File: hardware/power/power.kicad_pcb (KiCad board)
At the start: 2 copper layers, 37 x 41 mm, 30 parts, among them J1 SF6, J2 SF6, J3 PinHeader2x4, J4 PinHeader2x4, J5 PinHeader2x4, J6 SF6, J7 SF6, J8 SF6, Q1 ISC022N10NM6, Q2 ISC022N10NM6, Q3 ISC022N10NM6, Q4 ISC022N10NM6, Q5 ISC022N10NM6, Q6 ISC022N10NM6

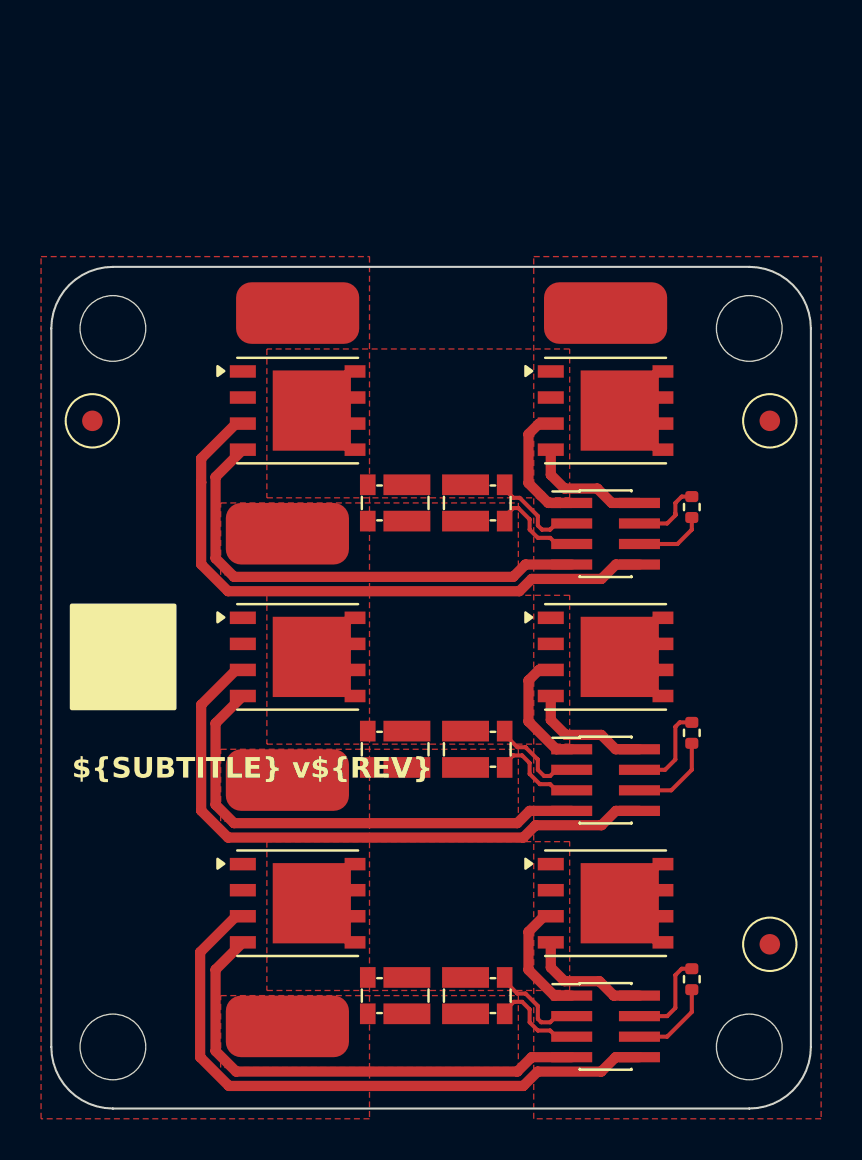
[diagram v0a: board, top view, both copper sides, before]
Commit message: intermediate commit, some changes needed before first purchase
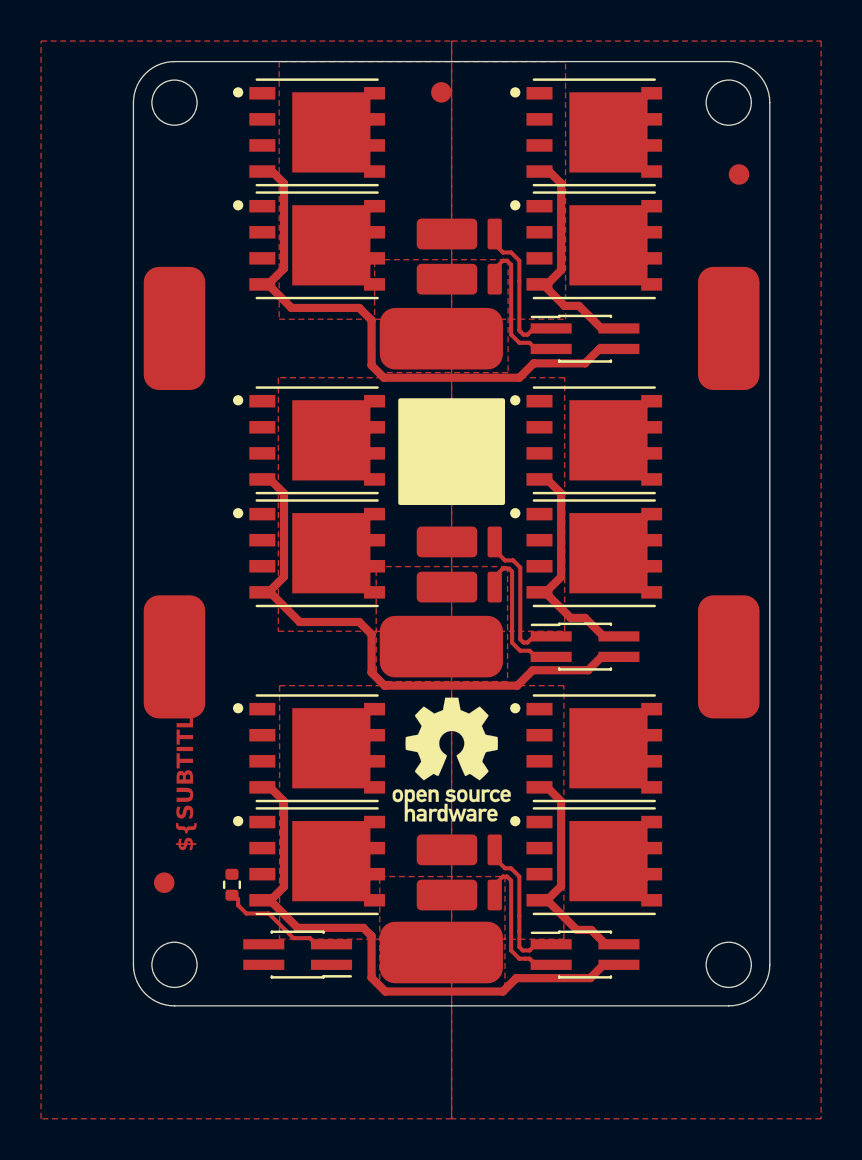
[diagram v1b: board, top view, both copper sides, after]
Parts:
- removed H1, H2, H3, H4: HoleM3_ISO14580, MountingHole:MountingHole_3.2mm_M3_ISO14580
- removed Q1, Q2, Q3, Q4, Q5, Q6: ISC022N10NM6, Package_SO:PowerPAK_SO-8_Single
- removed R2, R3, R4, R5, R6: 500u, Resistor_SMD:R_Shunt_Vishay_WSKW0612
- removed TH1, TH2, TH3: NTC 10k, Resistor_SMD:R_0402_1005Metric
- added H101: HoleM2_ISO14580, MountingHole:MountingHole_2.2mm_M2_ISO14580, F.Cu at (116.0, 42.0)
- added H102: HoleM2_ISO14580, MountingHole:MountingHole_2.2mm_M2_ISO14580, F.Cu at (89.0, 84.0)
- added H103: HoleM2_ISO14580, MountingHole:MountingHole_2.2mm_M2_ISO14580, F.Cu at (89.0, 42.0)
- added H104: HoleM2_ISO14580, MountingHole:MountingHole_2.2mm_M2_ISO14580, F.Cu at (116.0, 84.0)
- added J109: SF6, Connector_Wire:SolderWirePad_1x01_SMD_3x6mm, F.Cu at (116.0, 69.0)
- added J110: SF6, Connector_Wire:SolderWirePad_1x01_SMD_3x6mm, F.Cu at (89.0, 69.0)
- added J111: PinHeader2x2, Connector_PinHeader_1.00mm:PinHeader_2x02_P1.00mm_Vertical_SMD, F.Cu at (95.0, 83.5)
- added Q201: ISC022N10NM6, mcrmv:PowerPAK_SO-8_Single, F.Cu at (110.0, 43.5)
- added Q202: ISC022N10NM6, mcrmv:PowerPAK_SO-8_Single, F.Cu at (96.5, 43.5)
- added Q203: ISC022N10NM6, mcrmv:PowerPAK_SO-8_Single, F.Cu at (110.0, 58.5)
- added Q204: ISC022N10NM6, mcrmv:PowerPAK_SO-8_Single, F.Cu at (96.5, 58.5)
- added Q205: ISC022N10NM6, mcrmv:PowerPAK_SO-8_Single, F.Cu at (110.0, 73.5)
- added Q206: ISC022N10NM6, mcrmv:PowerPAK_SO-8_Single, F.Cu at (96.5, 73.5)
- added Q301: ISC022N10NM6, mcrmv:PowerPAK_SO-8_Single, F.Cu at (110.0, 49.0)
- added Q302: ISC022N10NM6, mcrmv:PowerPAK_SO-8_Single, F.Cu at (96.5, 49.0)
- added Q303: ISC022N10NM6, mcrmv:PowerPAK_SO-8_Single, F.Cu at (110.0, 64.0)
- added Q304: ISC022N10NM6, mcrmv:PowerPAK_SO-8_Single, F.Cu at (96.5, 64.0)
- added Q305: ISC022N10NM6, mcrmv:PowerPAK_SO-8_Single, F.Cu at (110.0, 79.0)
- added Q306: ISC022N10NM6, mcrmv:PowerPAK_SO-8_Single, F.Cu at (96.5, 79.0)
- added R102: 200u, mcrmv:WSK1216, F.Cu at (104.0, 64.5)
- added R103: 200u, mcrmv:WSK1216, F.Cu at (104.0, 79.5)
- added REF**: OSHW-Logo_5.7x6mm_SilkScreen, Symbol:OSHW-Logo_5.7x6mm_SilkScreen, F.Cu at (102.5, 74.0)
- added TH101: NTC 10k, Resistor_SMD:R_0402_1005Metric, F.Cu at (91.8, 80.1)
- J103: renamed from J3; value PinHeader2x4 -> PinHeader2x2; footprint Connector_PinHeader_1.00mm:PinHeader_2x04_P1.00mm_Vertical_SMD -> Connector_PinHeader_1.00mm:PinHeader_2x02_P1.00mm_Vertical_SMD
- J104: renamed from J4; value PinHeader2x4 -> PinHeader2x2; footprint Connector_PinHeader_1.00mm:PinHeader_2x04_P1.00mm_Vertical_SMD -> Connector_PinHeader_1.00mm:PinHeader_2x02_P1.00mm_Vertical_SMD
- J105: renamed from J5; value PinHeader2x4 -> PinHeader2x2; footprint Connector_PinHeader_1.00mm:PinHeader_2x04_P1.00mm_Vertical_SMD -> Connector_PinHeader_1.00mm:PinHeader_2x02_P1.00mm_Vertical_SMD
- R101: renamed from R1; value 500u -> 200u; footprint Resistor_SMD:R_Shunt_Vishay_WSKW0612 -> mcrmv:WSK1216
- moved FID101 33.7 mm to (116.5, 45.5)
- moved FID102 29.7 mm to (88.5, 80.0)
- moved FID103 22.6 mm to (102.0, 41.5)
- moved J106 12.1 mm to (102.0, 53.5)
- moved R101 12.0 mm to (104.0, 49.5), turned to 180 degrees
- moved J107 9.92 mm to (102.0, 68.5)
- moved J103 9.55 mm to (109.0, 53.5)
- moved J108 8.32 mm to (102.0, 83.4)
- moved J104 6.58 mm to (109.0, 68.5)
- moved J101 6.05 mm to (116.0, 53.0), turned to 180 degrees
- moved J102 6.05 mm to (89.0, 53.0), turned to 180 degrees
- moved J105 3.64 mm to (109.0, 83.5)
- renumbered FID1 to FID101, FID2 to FID102, FID3 to FID103, J1 to J101, J2 to J102, J6 to J106, J7 to J107, J8 to J108
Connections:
- J103 pad 1: /P1 -> /S1_P
- J103 pad 3: /S1_P -> /S1_N
- J103 pad 4: /NTC1+ -> /GL1
- J104 pad 1: /P2 -> /S2_P
- J104 pad 3: /S2_P -> /S2_N
- J104 pad 4: /NTC2+ -> /GL2
- J105 pad 1: /P3 -> /S3_P
- J105 pad 3: /S3_P -> /S3_N
- J105 pad 4: /NTC3+ -> /GL3
- R101 pad 1: /P1 -> /P1_TAB
- R101 pad 2: /S1_P -> /S1_N
- R101 pad 3: /S1_N -> /S1_P
- R101 pad 4: /P1_TAB -> /P1
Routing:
- net GND: track 91.1 -> 0.00 mm
- net /P1: track 6.19 -> 0.00 mm
- net /P2: track 5.96 -> 0.00 mm
- net /P3: track 5.88 -> 0.00 mm
- net /GH1: track 6.11 -> 11.6 mm
- net /GH3: track 6.11 -> 11.6 mm
- net /GH2: track 6.08 -> 11.5 mm
- net /NTC3+: track 4.44 -> 0.00 mm
- net /NTC2+: track 4.44 -> 0.00 mm
- net /NTC2-: track 4.25 -> 0.00 mm
- net /NTC3-: track 4.14 -> 0.00 mm
- net /GL1: track 23.8 -> 27.9 mm
- net /GL3: track 23.9 -> 27.8 mm
- net /GL2: track 23.8 -> 27.7 mm
- net /NTC1-: track 3.43 -> 0.00 mm
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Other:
- board size 37 x 41 mm -> 31 x 46 mm
- board text added: "${TITLE} ${SUBTITLE} 2025"
- board text removed: "${TITLE} ${SUBTITLE} v${REV}"
